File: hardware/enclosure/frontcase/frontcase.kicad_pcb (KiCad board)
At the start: 2 copper layers, 42.5 x 23 mm, 1 part

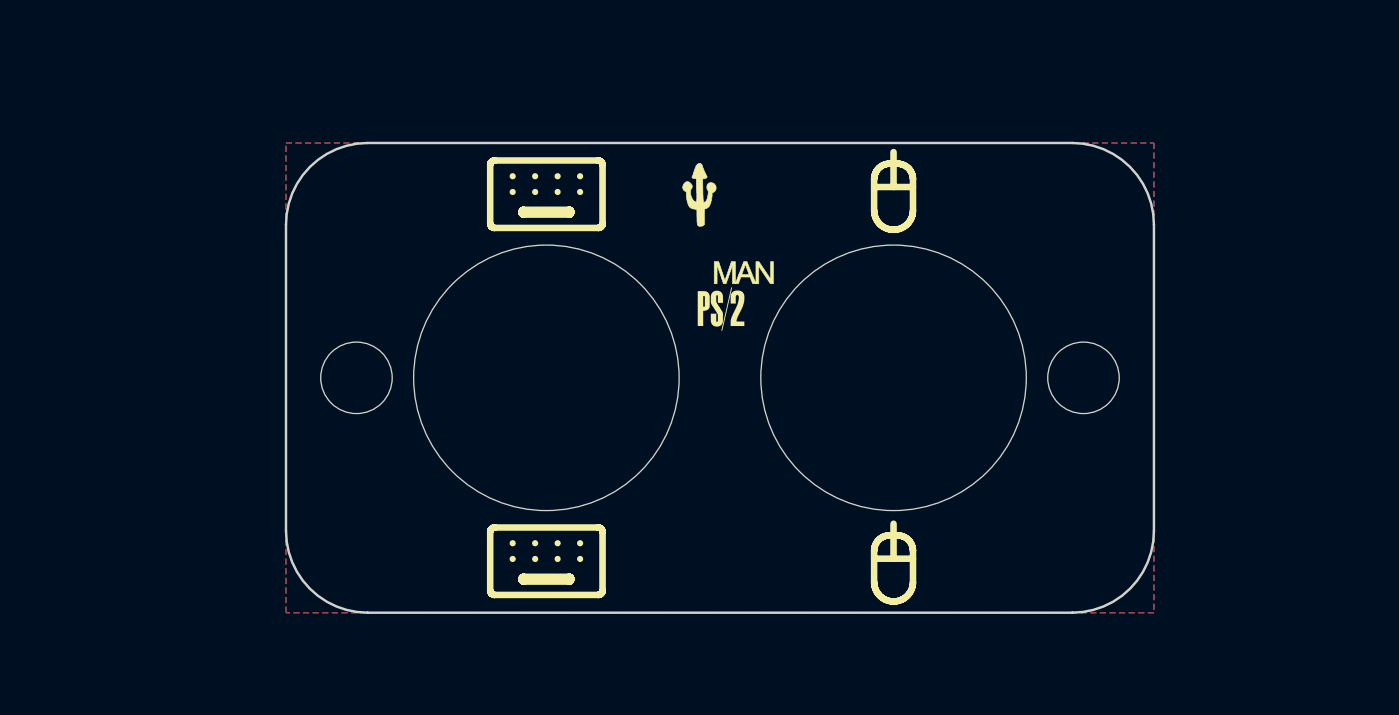
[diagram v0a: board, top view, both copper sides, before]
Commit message: serial enclosure
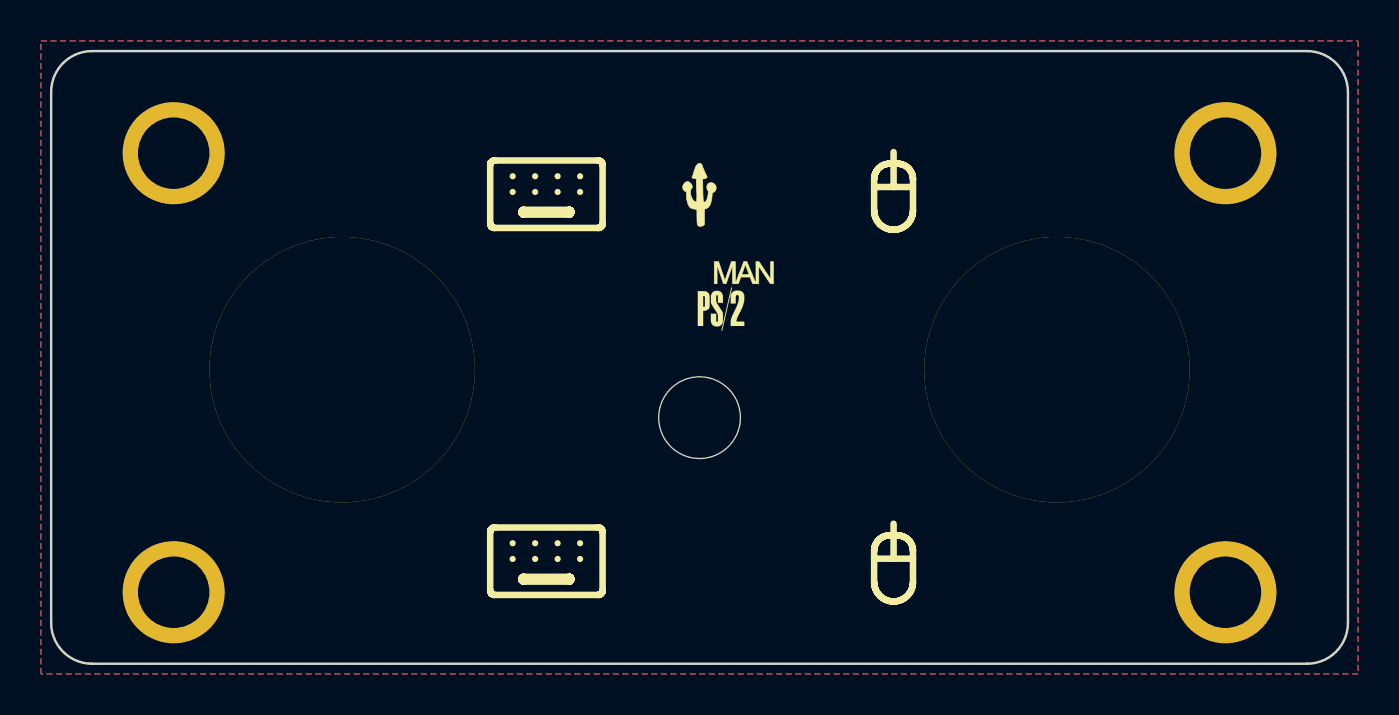
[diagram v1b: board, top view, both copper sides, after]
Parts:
- moved REF** 1.41 mm to (144.0, 96.0)
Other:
- board size 42.5 x 23 mm -> 63.5 x 30 mm
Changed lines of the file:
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@@
   (net 0 "")
   (footprint "ps2usb:frontpanel" (layer "F.Cu")
-    (at 145 97)
+    (at 144 96)
     (attr through_hole)
     (fp_text reference "REF**" (at 0 -0.5 unlocked) (layer "F.SilkS") hide
@@
       (effects (font (size 1 1) (thickness 0.15)))
     )
-    (fp_line (start 21.25 7.5) (end 21.25 -7.5) (layer "Edge.Cuts") (width 0.12))
-    (fp_line (start 17.25 11.5) (end -17.25 11.5) (layer "Edge.Cuts") (width 0.12))
-    (fp_line (start -21.25 7.5) (end -21.25 -7.5) (layer "Edge.Cuts") (width 0.12))
-    (fp_line (start -17.25 -11.5) (end 17.25 -11.5) (layer "Edge.Cuts") (width 0.12))
-    (fp_arc (start -21.25 -7.5) (mid -20.078427 -10.328427) (end -17.25 -11.5) (layer "Edge.Cuts") (width 0.12))
-    (fp_arc (start 17.25 -11.5) (mid 20.078427 -10.328427) (end 21.25 -7.5) (layer "Edge.Cuts") (width 0.12))
-    (fp_arc (start 21.25 7.5) (mid 20.078427 10.328427) (end 17.25 11.5) (layer "Edge.Cuts") (width 0.12))
-    (fp_arc (start -17.25 11.5) (mid -20.078427 10.328427) (end -21.25 7.5) (layer "Edge.Cuts") (width 0.12))
-    (pad "" np_thru_hole circle (at 8.5 0) (size 13 13) (drill 13) (layers F&B.Cu *.Mask))
-    (pad "" np_thru_hole circle (at 17.8 0) (size 3.5 3.5) (drill 3.5) (layers F&B.Cu *.Mask)
-      (clearance 1))
-    (pad "" np_thru_hole circle (at -17.8 0) (size 3.5 3.5) (drill 3.5) (layers F&B.Cu *.Mask)
-      (clearance 1))
-    (pad "" np_thru_hole circle (at -8.5 0) (size 13 13) (drill 13) (layers F&B.Cu *.Mask))
+    (fp_line (start -31.75 13) (end -31.75 -13) (layer "Edge.Cuts") (width 0.12))
+    (fp_line (start 29.75 15) (end -29.75 15) (layer "Edge.Cuts") (width 0.12))
+    (fp_line (start 31.75 13) (end 31.75 -13) (layer "Edge.Cuts") (width 0.12))
+    (fp_line (start -29.75 -15) (end 29.75 -15) (layer "Edge.Cuts") (width 0.12))
+    (fp_arc (start -31.75 -13) (mid -31.164214 -14.414214) (end -29.75 -15) (layer "Edge.Cuts") (width 0.12))
+    (fp_arc (start 29.75 -15) (mid 31.164214 -14.414214) (end 31.75 -13) (layer "Edge.Cuts") (width 0.12))
+    (fp_arc (start -29.75 15) (mid -31.164214 14.414214) (end -31.75 13) (layer "Edge.Cuts") (width 0.12))
+    (fp_arc (start 31.75 13) (mid 31.164214 14.414214) (end 29.75 15) (layer "Edge.Cuts") (width 0.12))
+    (pad "" np_thru_hole circle (at 0 2.95) (size 4 4) (drill 4) (layers F&B.Cu *.Mask))
+    (pad "1" thru_hole circle (at -25.75 11.5) (size 5 5) (drill 3.5) (layers *.Cu *.Mask))
+    (pad "1" thru_hole circle (at 25.75 -10) (size 5 5) (drill 3.5) (layers *.Cu *.Mask))
+    (pad "1" thru_hole circle (at -25.75 -10) (size 5 5) (drill 3.5) (layers *.Cu *.Mask))
+    (pad "1" thru_hole circle (at 25.75 11.5) (size 5 5) (drill 3.5) (layers *.Cu *.Mask))
+    (pad "2" thru_hole circle (at -17.5 0.6) (size 13 13) (drill 13) (layers *.Cu *.Mask))
+    (pad "2" thru_hole circle (at 17.5 0.6) (size 13 13) (drill 13) (layers *.Cu *.Mask))
   )
   (gr_line (start 135.393669 106.96999) (end 135.388079 106.969565) (layer "F.SilkS") (width 0.333132))
@@
   (gr_line (start 137.674673 88.971407) (end 137.670679 88.974866) (layer "F.SilkS") (width 0.333132))
   (gr_line (start 153.597551 89.745105) (end 153.549106 89.748766) (layer "F.SilkS") (width 0.32))
-  (gr_rect (start 123.75 85.5) (end 166.25 108.5) (layer "B.Mask") (width 0.15) (fill solid))
+  (gr_rect (start 111.75 80.5) (end 176.25 111.5) (layer "B.Mask") (width 0.15) (fill solid))
   (gr_poly
     (pts
@@
     (polygon
       (pts
-        (xy 166.25 108.5)
-        (xy 123.75 108.5)
-        (xy 123.75 85.5)
-        (xy 166.25 85.5)
+        (xy 176.25 111.5)
+        (xy 111.75 111.5)
+        (xy 111.75 80.5)
+        (xy 176.25 80.5)
       )
     )
@@
     (polygon
       (pts
-        (xy 166.245386 108.498846)
-        (xy 123.745386 108.498846)
-        (xy 123.745386 85.498846)
-        (xy 166.245386 85.498846)
+        (xy 176.245386 111.498846)
+        (xy 111.745386 111.498846)
+        (xy 111.745386 80.498846)
+        (xy 176.245386 80.498846)
       )
     )
